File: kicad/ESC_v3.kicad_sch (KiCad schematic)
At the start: 26 parts, among them J1 Conn_01x05_Pin, J2 Conn_01x05_Pin, J3 Conn_01x03_Pin, J4 Conn_01x06_Pin, J5 Conn_01x02_Pin, J6 Conn_01x06_Pin, J7 Conn_01x02_Pin, J8 Conn_01x04_Pin, SW2 SW_Nidec_CAS-120A1, U1 STSPIN32G4, U10 BD4104, U14 MCP9700x-ETT

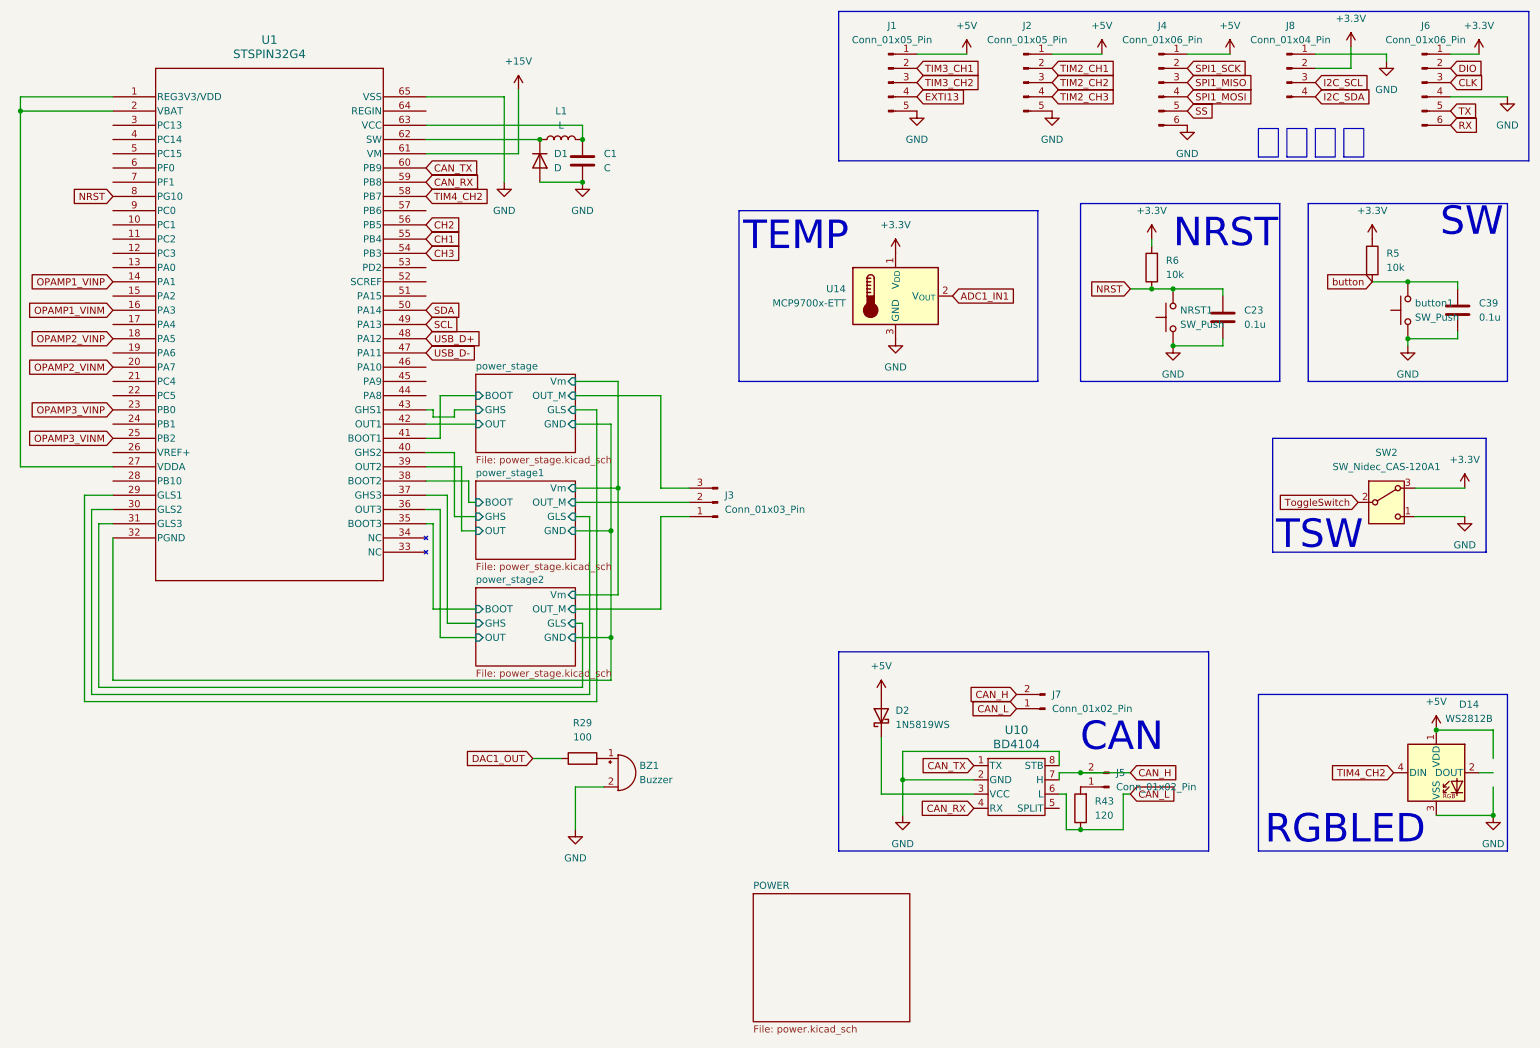
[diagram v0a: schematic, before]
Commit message: a
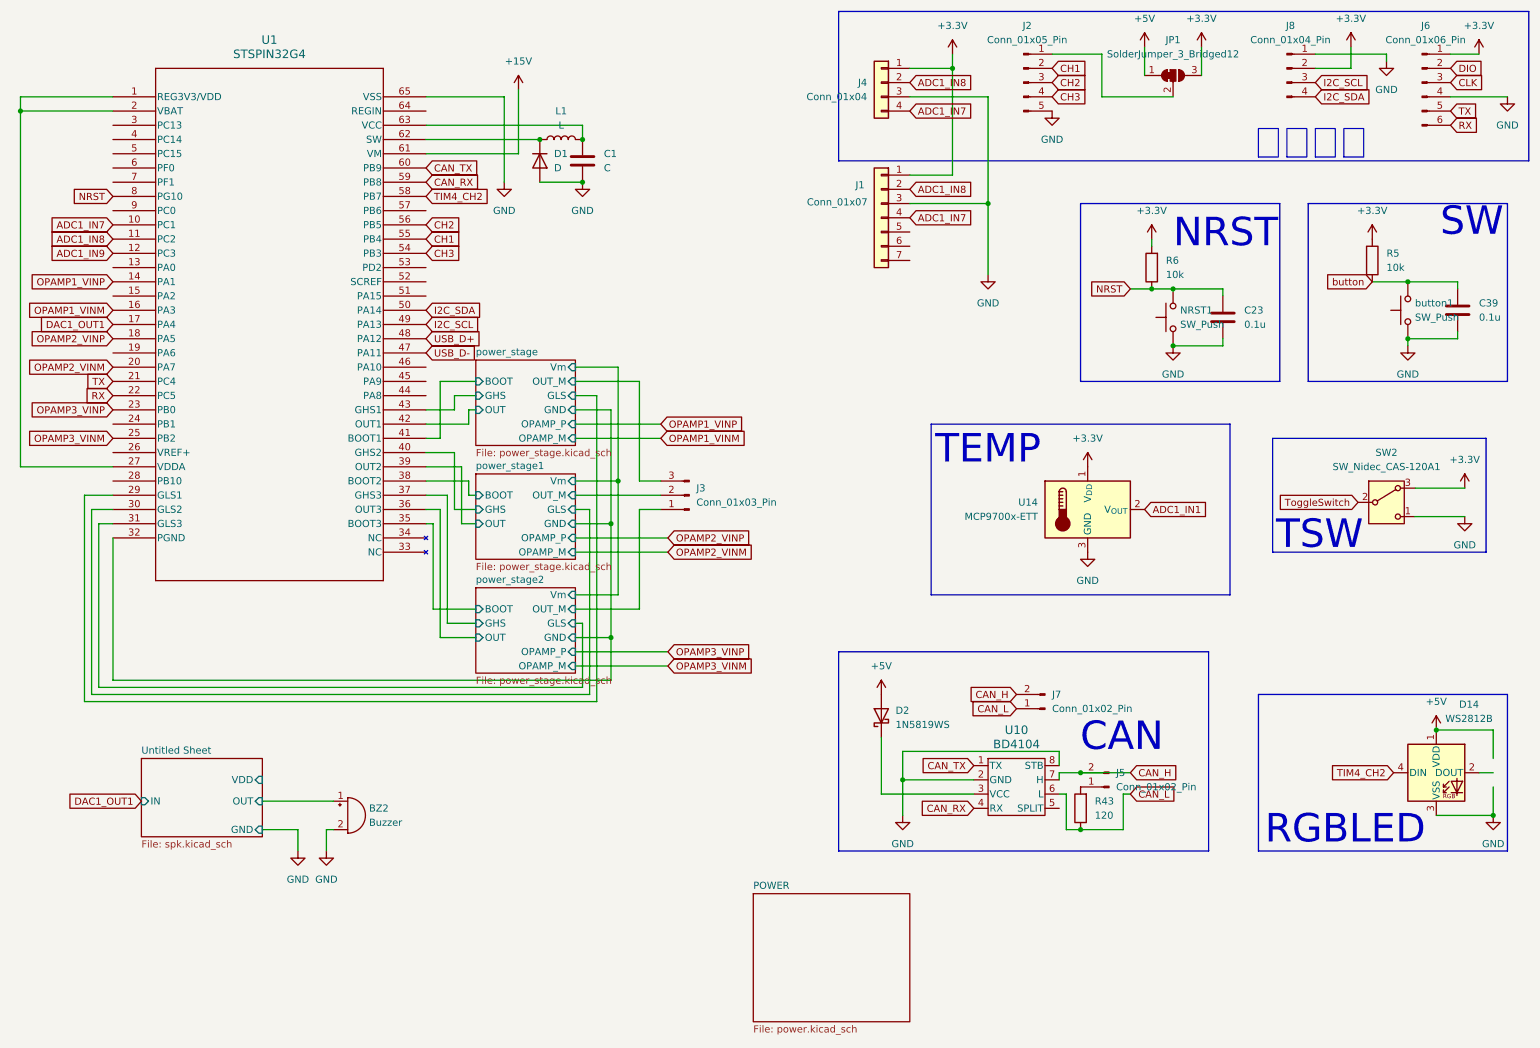
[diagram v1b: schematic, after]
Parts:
- removed BZ1: Buzzer, jisaku:buzzer_unified, symbol Device:Buzzer
- removed J1: Conn_01x05_Pin, Connector_JST:JST_XH_S5B-XH-A_1x05_P2.50mm_Horizontal, symbol Connector:Conn_01x05_Pin
- removed J4: Conn_01x06_Pin, Connector_JST:JST_PH_B6B-PH-K_1x06_P2.00mm_Vertical, symbol Connector:Conn_01x06_Pin
- removed R29: 100, Resistor_SMD:R_0402_1005Metric_Pad0.72x0.64mm_HandSolder, symbol Device:R
- added BZ2: Buzzer, jisaku:buzzer_unified, symbol Device:Buzzer
- added J1: Conn_01x07, Connector_JST:JST_GH_SM07B-GHS-TB_1x07-1MP_P1.25mm_Horizontal, symbol Connector_Generic:Conn_01x07
- added J4: Conn_01x04, Connector_JST:JST_GH_SM04B-GHS-TB_1x04-1MP_P1.25mm_Horizontal, symbol Connector_Generic:Conn_01x04
- added JP1: SolderJumper_3_Bridged12, symbol Jumper:SolderJumper_3_Bridged12
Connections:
- net SCL is gone; now on net I2C_SCL: U1.49 (PA13)
- net SDA is gone; now on net I2C_SDA: U1.50 (PA14)
- net TIM2_CH1 is gone; now on net CH1: J2.2 (Pin_2)
- net TIM2_CH2 is gone; now on net CH2: J2.3 (Pin_3)
- net TIM2_CH3 is gone; now on net CH3: J2.4 (Pin_4)
- net +3.3V: now also J1.1 (Pin_1), J4.1 (Pin_1), JP1.3 (B)
- net +5V: now also JP1.1 (A); no longer J2.1 (Pin_1)
- net GND: now also BZ2.2 (-), J1.3 (Pin_3), J4.3 (Pin_3)
- net RX: now also U1.22 (PC5)
- net TX: now also U1.21 (PC4)
- net ADC1_IN7: now reaches U1.10 (PC1)
- net ADC1_IN7: now also J1.4 (Pin_4), J4.4 (Pin_4)
- net ADC1_IN8: now reaches U1.11 (PC2)
- net ADC1_IN8: now also J1.2 (Pin_2), J4.2 (Pin_2)
- net ADC1_IN9: now reaches U1.12 (PC3)
- net DAC1_OUT1: now reaches U1.17 (PA4)
- new net: J2.1 (Pin_1), JP1.2 (C)
- new net Untitled Sheet/OUT: BZ2.1 (+)
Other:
- added sheet Untitled Sheet (spk.kicad_sch)
- sheet power_stage ports: added OPAMP_M, OPAMP_P; removed none
- sheet power_stage1 ports: added OPAMP_M, OPAMP_P; removed none
- sheet power_stage2 ports: added OPAMP_M, OPAMP_P; removed none
- moved on the sheet: J3, U14
